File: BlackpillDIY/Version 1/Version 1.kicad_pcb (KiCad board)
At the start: 2 copper layers, 78 x 39.1 mm, 39 parts, among them J1 Conn_01x08, J2 Conn_01x08, J3 Debug, J4 Left Header, J5 Right Header, J6 Conn_01x05, J7 Conn_01x05, J8 Conn_01x05, J9 Conn_01x08, U1 HT-CT62, U2 STM32F411CCUx, U3 SAM-M8Q, U4 LIS2MDL, Y1 LFXTAL062558Reel, Y2 Crystal_GND24

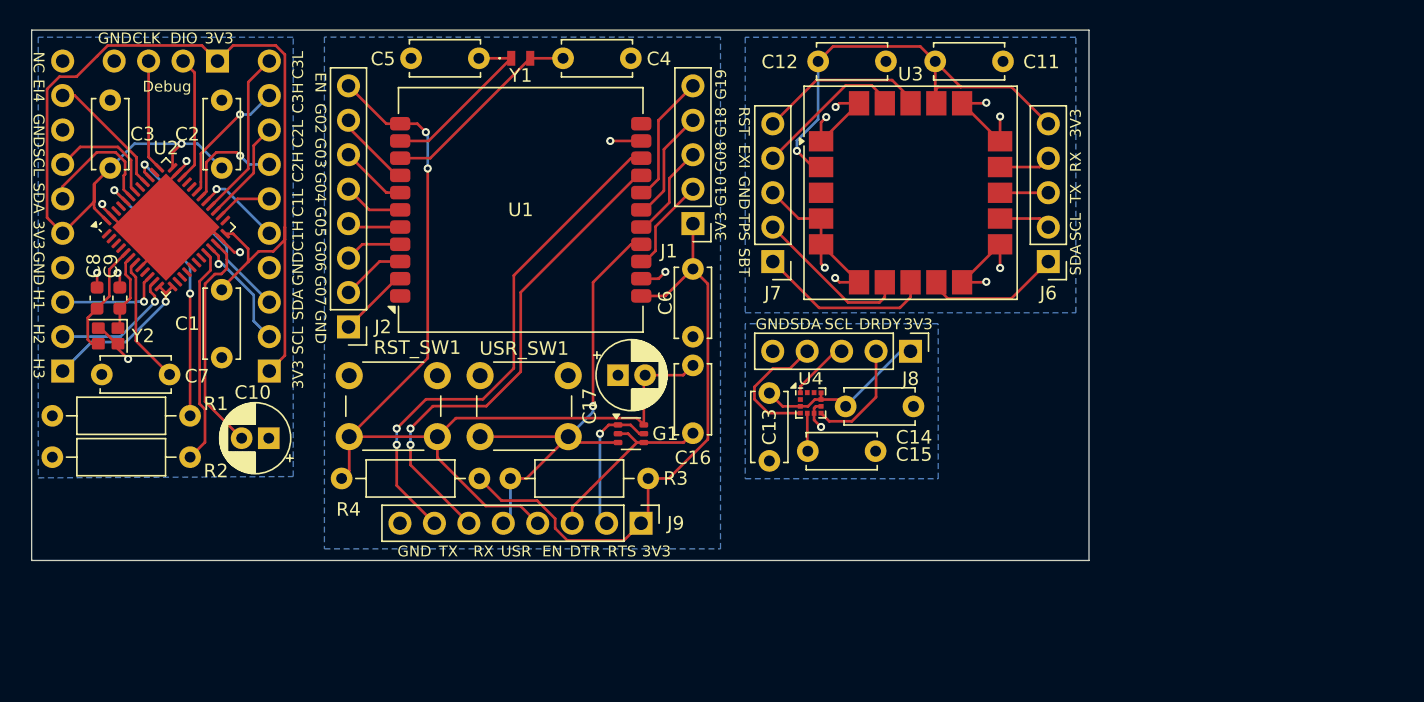
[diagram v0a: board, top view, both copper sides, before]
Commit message: board breaks
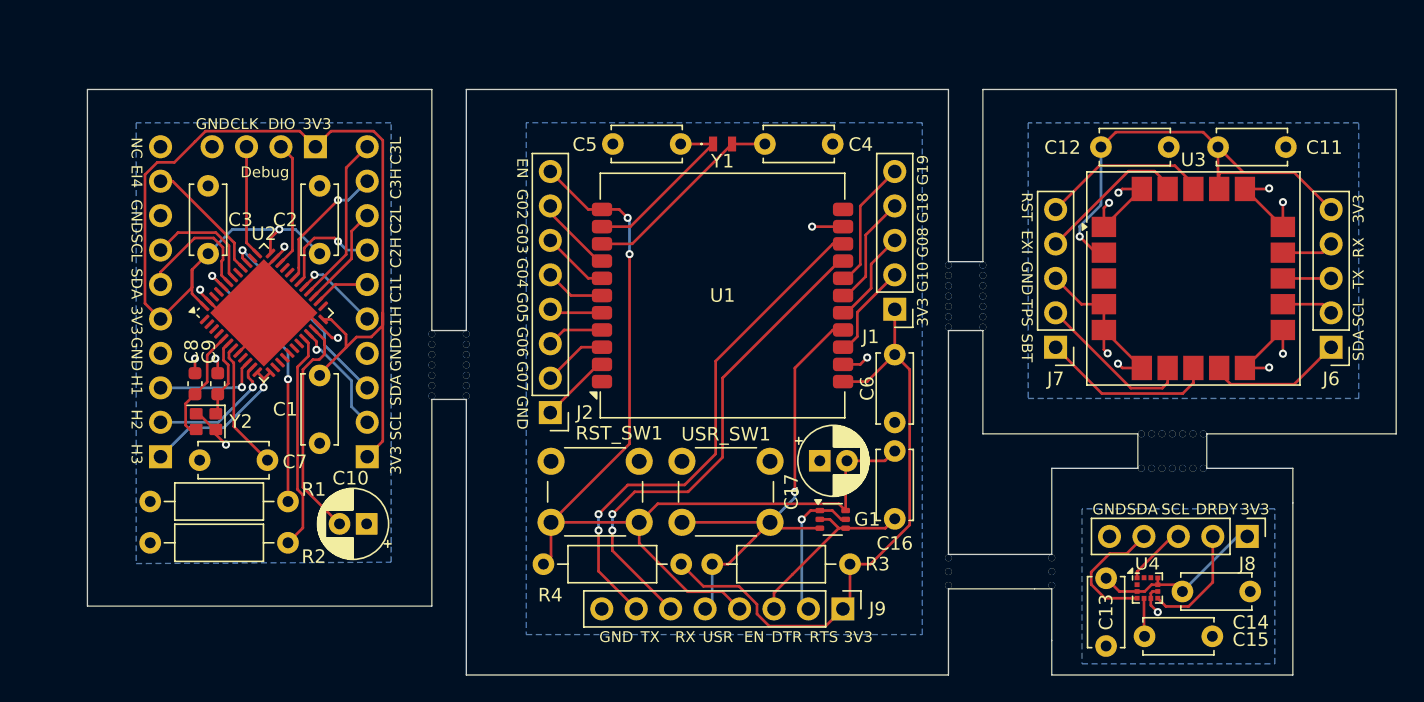
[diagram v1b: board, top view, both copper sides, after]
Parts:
- moved J8 28.3 mm to (103.3, 50.7)
- moved C13 28.3 mm to (92.9, 53.8)
- moved C14 28.3 mm to (98.5, 54.8)
- moved C15 28.3 mm to (95.7, 58.1)
- moved U4 28.3 mm to (96.0, 54.6)
- moved J7 21.8 mm to (89.2, 36.8)
- moved U3 21.8 mm to (99.3, 31.7)
- moved C11 21.8 mm to (101.2, 22.0)
- moved C12 21.8 mm to (92.5, 22.0)
- moved J6 21.8 mm to (109.5, 36.8)
- moved C4 16.2 mm to (67.7, 21.8)
- moved C5 16.2 mm to (61.5, 21.8)
- moved J2 16.2 mm to (51.9, 41.6)
- moved Y1 16.2 mm to (64.6, 21.8)
- moved C16 16.2 mm to (77.3, 49.4)
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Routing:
- net (no net): vias 0 -> 48
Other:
- board size 78 x 39.1 mm -> 96.5 x 43.2 mm
